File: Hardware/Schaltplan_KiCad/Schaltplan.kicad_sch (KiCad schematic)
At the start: 36 parts, among them J1 3-106505-2, J3 Conn_01x04_Pin, J4 Conn_01x02_Pin, U1 MCP2562-E-SN, U3 ESP32-DEVKITC-32U, U5 PCA9306DCTR

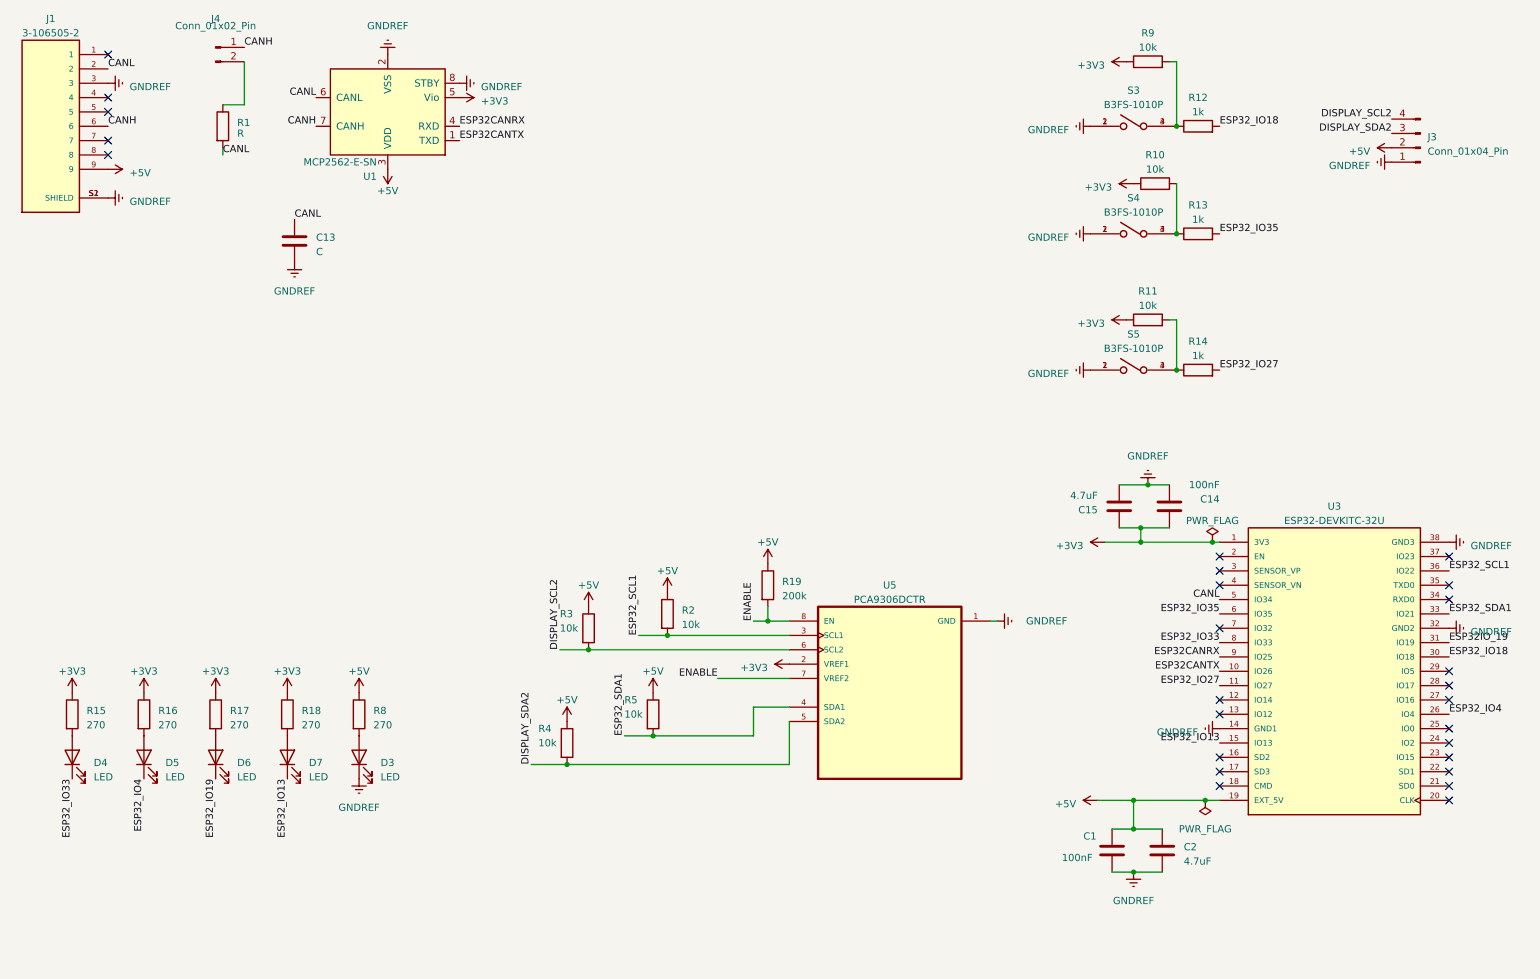
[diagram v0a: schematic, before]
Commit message: finishes PCB Design
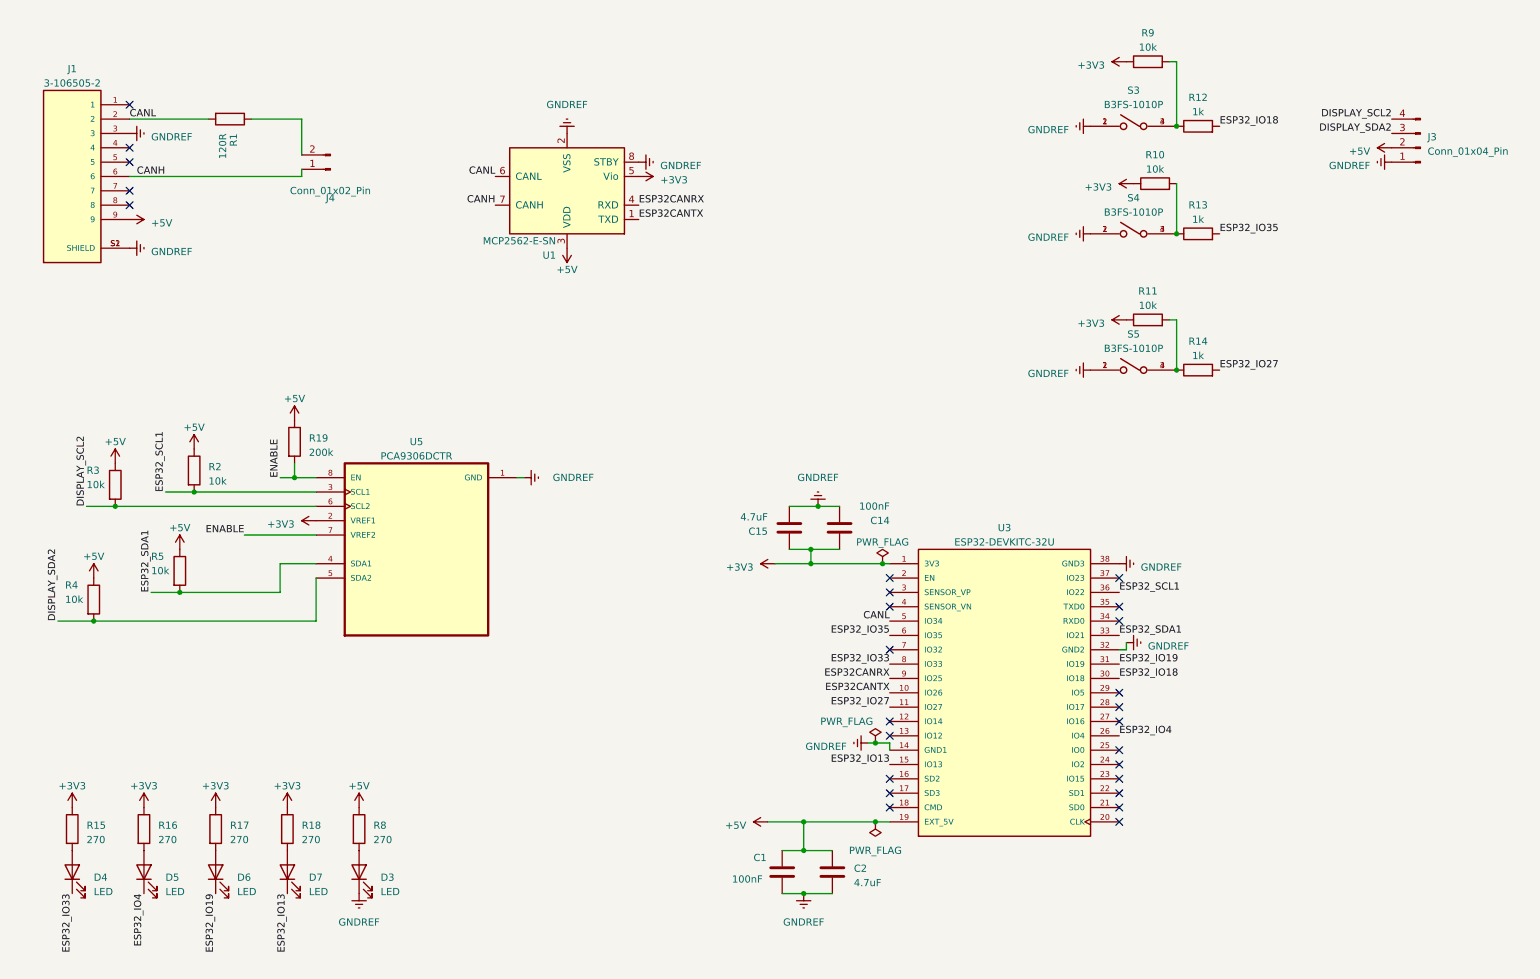
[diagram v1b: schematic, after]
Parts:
- removed C13: C, Capacitor_SMD:C_1812_4532Metric_Pad1.57x3.40mm_HandSolder, symbol Device:C
- C1, C14, C15, C2: footprint Capacitor_SMD:C_1812_4532Metric_Pad1.57x3.40mm_HandSolder -> Capacitor_SMD:C_0603_1608Metric_Pad1.08x0.95mm_HandSolder
- R1: value R -> 120R; footprint Resistor_SMD:R_2010_5025Metric_Pad1.40x2.65mm_HandSolder -> Resistor_SMD:R_0603_1608Metric_Pad0.98x0.95mm_HandSolder
- R10, R11, R12, R13, R14, R15, R16, R17, R18, R19, R2, R3, R4, R5, R8, R9: footprint Resistor_SMD:R_2010_5025Metric_Pad1.40x2.65mm_HandSolder -> Resistor_SMD:R_0603_1608Metric_Pad0.98x0.95mm_HandSolder
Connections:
- net ESP32IO_19 is gone; now on net ESP32_IO19: U3.31 (IO19)
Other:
- moved on the sheet: C1, C14, C15, C2, D3, D4, D5, D6, D7, J1, J4, R1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
